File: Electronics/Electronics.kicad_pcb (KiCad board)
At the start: 2 copper layers, 35 parts, among them J1 Barrel_Jack, M1 Fan_4pin, Q1 PN2222A, Q2 PN2222A, Q3 PN2222A, SW1 MOTOR_DECREASE, SW2 MOTOR_INCREASE, SW3 CYCLE_MODE, SW4 CYCLE_COLOR, SW5 SW_Wuerth_450301014042, U1 5VDC<-12VDC, U3 ESP32-DEVKIT-V1

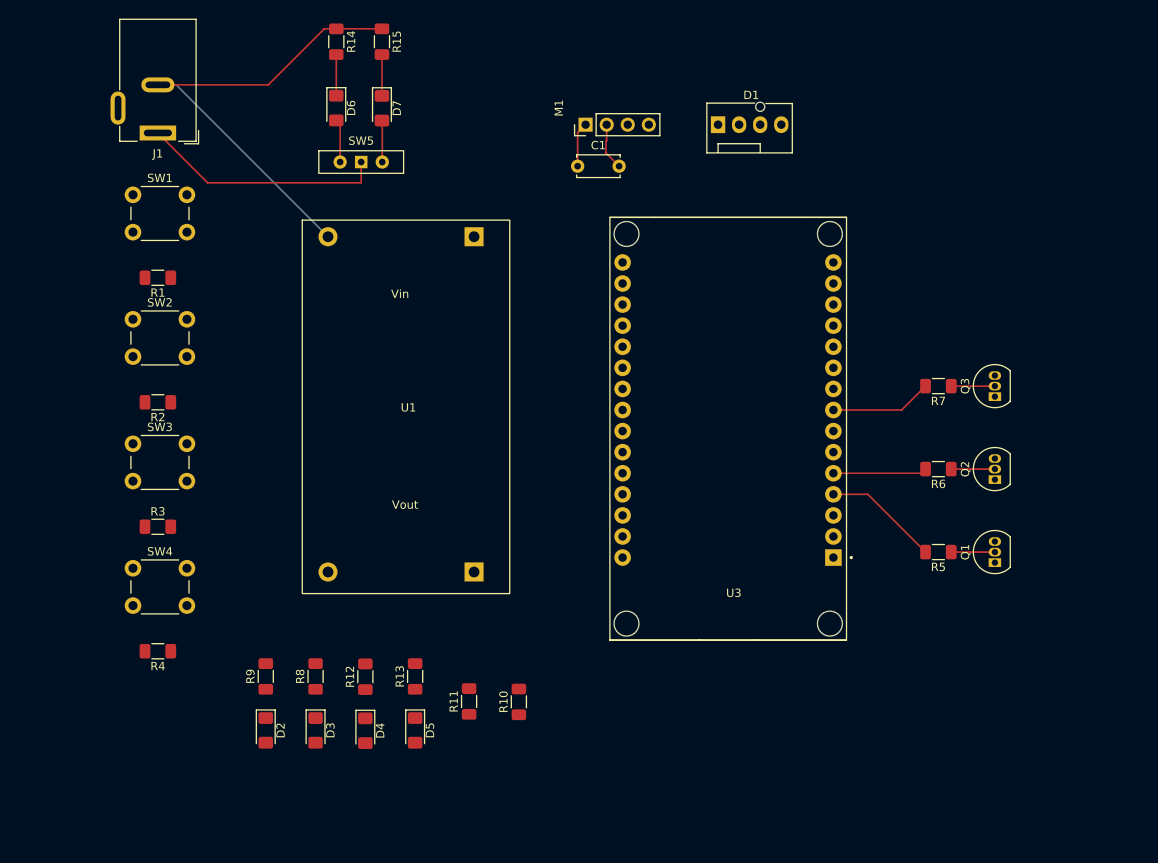
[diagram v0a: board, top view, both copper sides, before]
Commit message: Finalized. Awaiting PCB Production
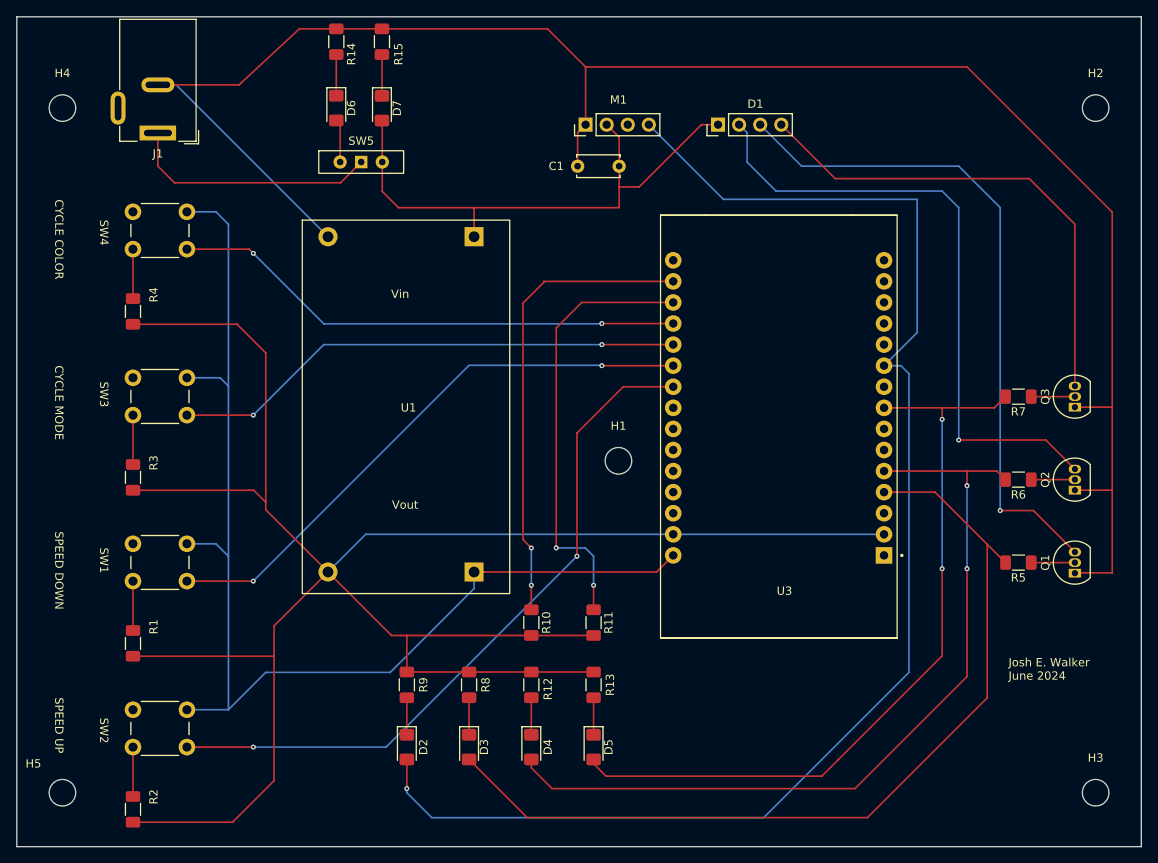
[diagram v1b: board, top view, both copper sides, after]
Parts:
- added H1: MountingHole, MountingHole:MountingHole_3.2mm_M3, F.Cu at (157.0, 107.0)
- added H2: MountingHole, MountingHole:MountingHole_3.2mm_M3, F.Cu at (214.5, 64.5)
- added H3: MountingHole, MountingHole:MountingHole_3.2mm_M3, F.Cu at (214.5, 147.0)
- added H4: MountingHole, MountingHole:MountingHole_3.2mm_M3, F.Cu at (90.0, 64.5)
- added H5: MountingHole, MountingHole:MountingHole_3.2mm_M3, F.Cu at (90.0, 147.0)
- D1: footprint Connector:FanPinHeader_1x04_P2.54mm_Vertical -> Connector_PinHeader_2.54mm:PinHeader_1x04_P2.54mm_Vertical
- U3: footprint ESP32_DEVKITV1:MODULE_ESP32_DEVKIT_V1 -> Custom:MODULE_ESP32_DEVKIT_V1_NO_MOUNT
- moved R2 49.1 mm to (98.5, 149.0), turned to -90 degrees
- moved SW2 47.0 mm to (98.5, 137.0)
- moved R1 44.2 mm to (98.5, 129.0), turned to 90 degrees
- moved SW4 43.0 mm to (98.5, 77.0)
- moved SW1 42.0 mm to (98.5, 117.0)
- moved R4 41.1 mm to (98.5, 89.0), turned to -90 degrees
- moved D5 21.6 mm to (154.0, 141.5)
- moved R13 21.5 mm to (154.0, 134.0)
- moved D4 20.1 mm to (146.5, 141.5)
- moved R12 20.0 mm to (146.5, 134.0)
- moved D3 18.6 mm to (139.0, 141.5)
- moved R8 18.5 mm to (139.0, 134.0)
- moved R11 17.8 mm to (154.0, 126.5), turned to -90 degrees
- moved D2 17.1 mm to (131.5, 141.5)
- moved R9 17.0 mm to (131.5, 134.0)
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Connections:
- C1 pad 1: GND -> GND_HIGH
- J1 pad 2: GND -> GND_HIGH
- M1 pad 1: GND -> GND_HIGH
- Q1 pad 1: GND -> GND_HIGH
- Q2 pad 1: GND -> GND_HIGH
- Q3 pad 1: GND -> GND_HIGH
- R1 pad 1: GND -> GND_LOW
- R10 pad 2: GND -> GND_LOW
- R11 pad 2: GND -> GND_LOW
- R12 pad 2: GND -> GND_LOW
- R13 pad 2: GND -> GND_LOW
- R14 pad 1: GND -> GND_HIGH
- R15 pad 1: GND -> GND_HIGH
- R2 pad 2: GND -> GND_LOW
- R3 pad 1: GND -> GND_LOW
- R4 pad 2: GND -> GND_LOW
- R8 pad 2: GND -> GND_LOW
- R9 pad 2: GND -> GND_LOW
- SW1 pad 1: Net-(U1-VOUT) -> unconnected-(SW1-Pad1)
- SW1 pad 2: unconnected-(SW1-Pad2) -> Net-(U1-VOUT)
- SW2 pad 1: Net-(U1-VOUT) -> unconnected-(SW2-Pad1)
- SW2 pad 2: unconnected-(SW2-Pad2) -> Net-(U1-VOUT)
- SW3 pad 1: Net-(U1-VOUT) -> unconnected-(SW3-Pad1)
- SW3 pad 2: unconnected-(SW3-Pad2) -> Net-(U1-VOUT)
- SW4 pad 1: Net-(U1-VOUT) -> unconnected-(SW4-Pad1)
- SW4 pad 2: unconnected-(SW4-Pad2) -> Net-(U1-VOUT)
- U1 pad 2: GND -> GND_HIGH
- U1 pad 4: GND -> GND_LOW
- U3 pad 2: GND -> GND_LOW
- U3 pad 29: GND -> GND_LOW
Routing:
- net GND_LOW: track 0.00 -> 258.4 mm
- net GND_HIGH: track 0.00 -> 214.7 mm
- net Net-(D2-A): track 0.00 -> 170.2 mm, vias 0 -> 1
- net Net-(U1-VOUT): track 0.00 -> 142.6 mm
- net Net-(D3-A): track 14.0 -> 108.0 mm
- net Net-(D4-A): track 11.3 -> 100.7 mm, vias 0 -> 2
- net Net-(SW2-K): track 0.00 -> 85.3 mm, vias 0 -> 2
- net Net-(D5-A): track 12.3 -> 94.2 mm, vias 0 -> 2
- net Net-(D1-RK): track 0.00 -> 80.6 mm, vias 0 -> 1
- net Net-(D1-GK): track 0.00 -> 76.1 mm, vias 0 -> 1
- net Net-(SW1-K): track 0.00 -> 69.4 mm, vias 0 -> 2
- net GND: track 63.3 -> 0.00 mm
- net Net-(SW4-K): track 0.00 -> 62.3 mm, vias 0 -> 2
- net Net-(SW3-K): track 0.00 -> 62.1 mm, vias 0 -> 2
- net Net-(D1-BK): track 0.00 -> 59.9 mm
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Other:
- board outline added: 135.5 x 100 mm
- board text added: "CYCLE COLOR"
- board text added: "CYCLE MODE"
- board text added: "Josh E. Walker June 2024"
- board text added: "SPEED DOWN"
- board text added: "SPEED UP"
